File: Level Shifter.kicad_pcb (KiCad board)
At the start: 2 copper layers, 36.6 x 27.9 mm, 15 parts, among them P1 3V3, P2 5V

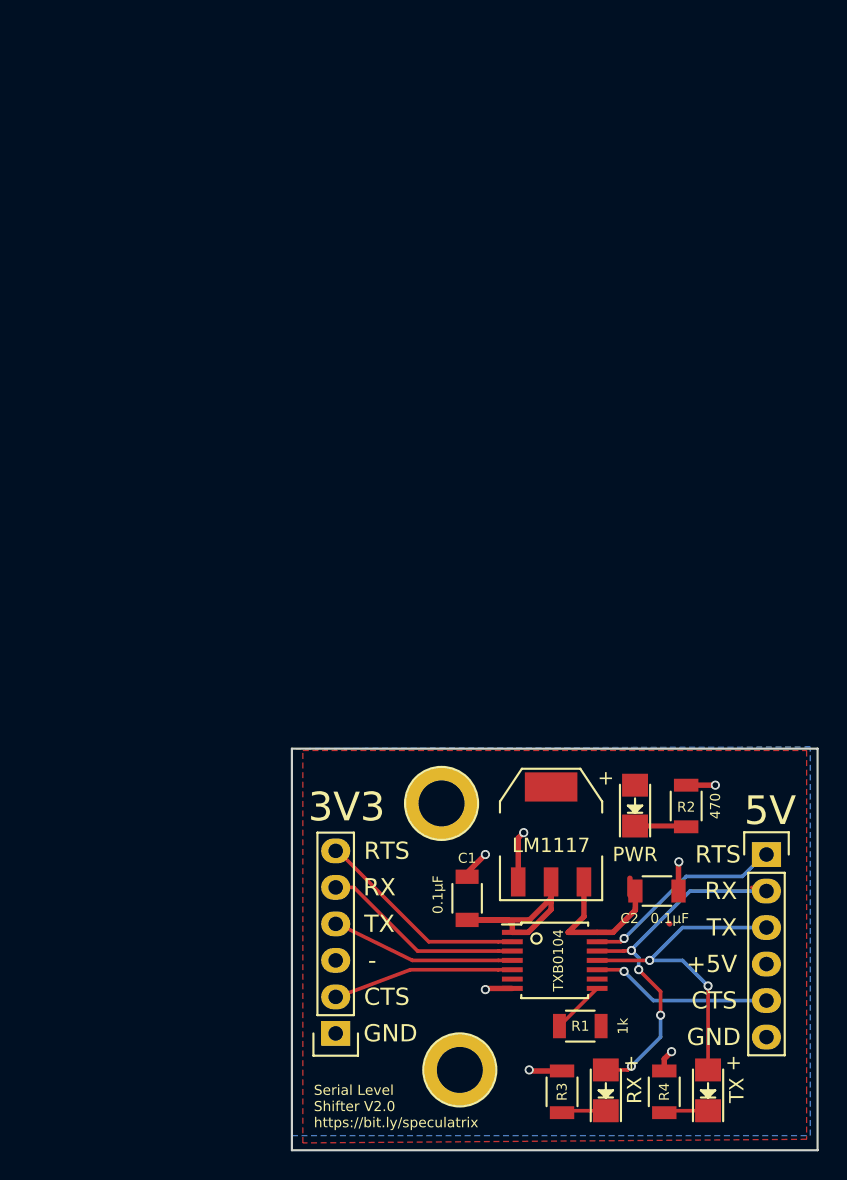
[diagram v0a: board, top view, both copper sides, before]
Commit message: Revised with fixes
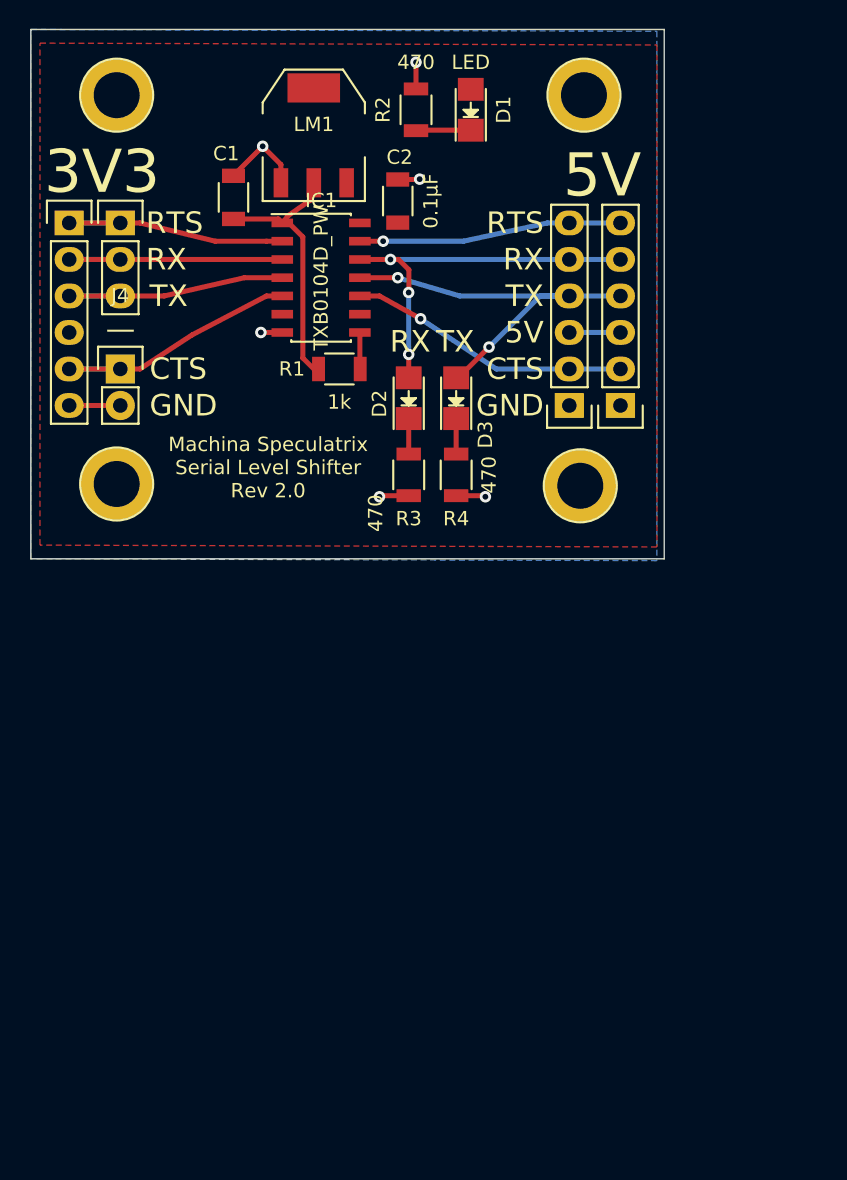
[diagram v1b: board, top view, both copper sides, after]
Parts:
- removed P1: 3V3, Pin_Headers:Pin_Header_Straight_1x06
- removed P2: 5V, Pin_Headers:Pin_Header_Straight_1x06
- removed the REF** at (162.6, 114.3)
- removed the REF** at (161.3, 95.8)
- removed TXB0104: TXB0104PW, Speculatrix_general:TSSOP-14_4.4x5mm_Pitch0.65mm_Pad0.35mm
- added IC1: TXB0104D_PW, Housings_SOIC:SOIC-14_3.9x8.7mm_Pitch1.27mm, F.Cu at (152.9, 59.2)
- added J1: 3V3, Pin_Headers:Pin_Header_Straight_1x06, F.Cu at (135.4, 55.4)
- added J2: 5V, Pin_Headers:Pin_Header_Straight_1x06, F.Cu at (173.7, 68.1)
- added J3: 3V3_test1, Pin_Headers:Pin_Header_Straight_1x03, F.Cu at (138.9, 55.4)
- added J4: 3V3_test2, Pin_Headers:Pin_Header_Straight_1x02, F.Cu at (138.9, 65.5)
- added J5: 5V_test, Pin_Headers:Pin_Header_Straight_1x06, F.Cu at (170.2, 68.1)
- added REF**: M3, Speculatrix_general:Mounting_hole_M3, F.Cu at (138.7, 73.5)
- added REF**: M3, Speculatrix_general:Mounting_hole_M3, F.Cu at (138.7, 46.5)
- added REF**: M3, Speculatrix_general:Mounting_hole_M3, F.Cu at (171.2, 46.5)
- added REF**: M3, Speculatrix_general:Mounting_hole_M3, F.Cu at (170.9, 73.7)
- D1: value PWR -> LED
- D2: value RX -> LED
- D3: value TX -> LED
- R3: value R3 -> 470
- R4: value R4 -> 470
- moved R2 52.0 mm to (159.5, 47.5)
- moved C1 51.4 mm to (146.8, 53.6)
- moved LM1 51.4 mm to (152.4, 49.3)
- moved C2 51.3 mm to (158.2, 53.8), turned to 90 degrees
- moved D3 51.2 mm to (162.3, 67.6)
- moved D2 50.1 mm to (159.0, 67.6)
- moved D1 49.7 mm to (163.3, 47.5)
- moved R1 48.7 mm to (154.2, 65.5), turned to 0 degrees
- moved R4 45.3 mm to (162.3, 72.9), turned to 270 degrees
- moved R3 44.2 mm to (159.0, 72.9), turned to 270 degrees
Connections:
- R1 pad 1: 5V -> 3V3
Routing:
- net /CTSH: track 12.7 -> 19.8 mm
- net /CTSL: track 12.6 -> 19.5 mm
- net /TXH: track 23.4 -> 29.1 mm
- net /TXL: track 12.9 -> 18.3 mm
- net 5V: track 11.9 -> 6.86 mm
- net /RTSH: track 14.3 -> 18.5 mm
- net /RXL: track 14.1 -> 18.1 mm
- net /RTSL: track 14.9 -> 18.3 mm
- net 3V3: track 16.1 -> 18.8 mm
- net GND: track 15.7 -> 18.3 mm, vias 7 -> 6
- net Net-(IC1-Pad8): track 3.71 -> 2.55 mm
- net /RXH: track 26.5 -> 27.6 mm, vias 4 -> 3
- net Net-(D2-Pad1): track 3.10 -> 2.46 mm
- net Net-(D3-Pad1): track 3.10 -> 2.46 mm
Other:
- board size 36.6 x 27.9 mm -> 44.1 x 36.8 mm
- net class Default: trace_width 0.254 -> 0.35; via_dia 0.635 -> 0.8; via_drill 0.381 -> 0.4
- net class power removed
- rule pad_to_mask_clearance: 0.2 -> 0
- board text added: "5V"
- board text added: "Machina Speculatrix Serial Level Shifter Rev 2.0"
- board text added: "—"
- board text removed: "+"
- board text removed: "+5V"
- board text removed: "-"
- board text removed: "Serial Level Shifter V2.0 https://bit.ly/speculatrix"
